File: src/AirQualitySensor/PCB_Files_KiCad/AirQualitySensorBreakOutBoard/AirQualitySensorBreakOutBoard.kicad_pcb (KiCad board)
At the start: 2 copper layers, 113.8 x 36 mm, 23 parts, among them J1 Conn_01x02_Male, J2 Conn_01x02_Male, J3 Conn_01x02_Male, J4 Conn_01x07_Male, Q1 IRLB8721PBF, U1 PMS5003, U2 PMS5003, U3 SPS30, U4 SHT31, U6 lilygo-ttgo-t-sim7000g-esp32-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

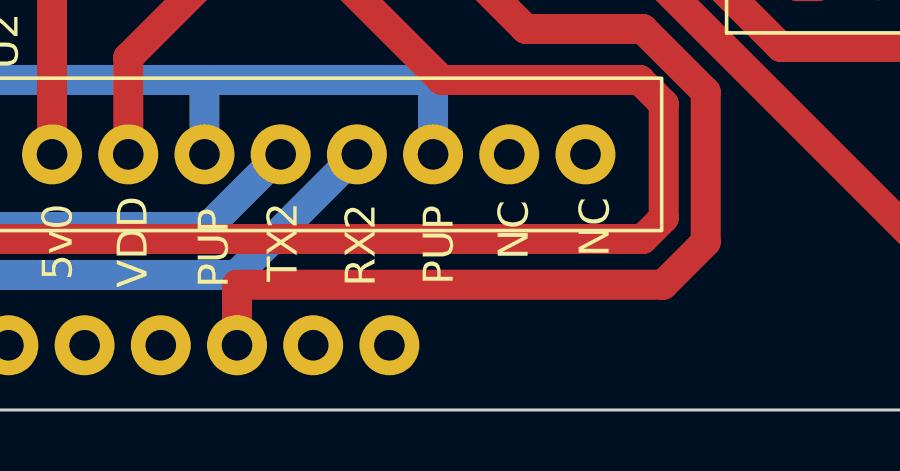
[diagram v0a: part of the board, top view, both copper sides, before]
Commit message: Fixed bug aqs
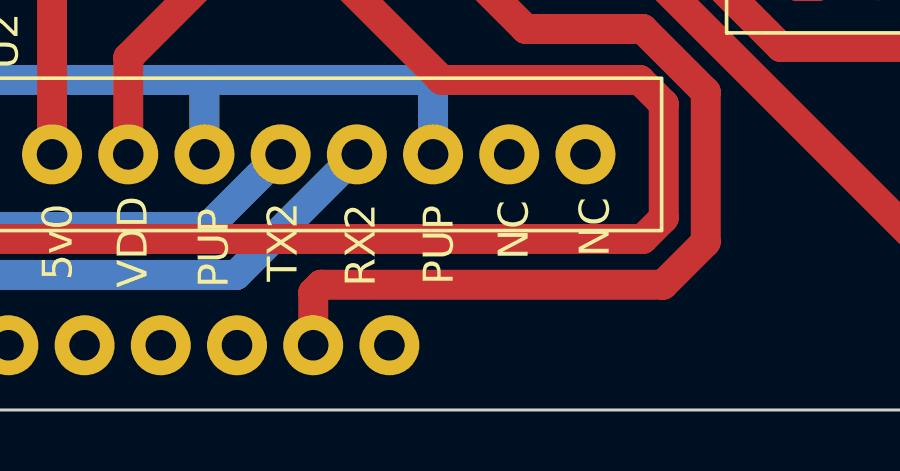
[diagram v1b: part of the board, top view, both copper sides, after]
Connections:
- U6 pad 12: unconnected-(U6-Pad12) -> VDD_EN
- U6 pad 13: VDD_EN -> unconnected-(U6-Pad13)
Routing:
- net VDD_EN: track 34.6 -> 31.9 mm
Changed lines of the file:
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@@
   (net 7 "unconnected-(U6-Pad03)")
   (net 8 "unconnected-(U6-Pad04)")
-  (net 9 "unconnected-(U6-Pad12)")
+  (net 9 "unconnected-(U6-Pad13)")
   (net 10 "unconnected-(U6-Pad14)")
   (net 11 "unconnected-(U6-Pad15)")
@@
       (net 34 "SPI_SS") (pinfunction "SPI__SS") (pintype "input"))
     (pad "12" thru_hole circle (at -14.12 -4.6 90) (size 2 2) (drill 1.02) (layers *.Cu *.Mask)
-      (net 9 "unconnected-(U6-Pad12)") (pinfunction "12") (pintype "input"))
+      (net 38 "VDD_EN") (pinfunction "12") (pintype "input"))
     (pad "13" thru_hole circle (at -14.12 -7.14 90) (size 2 2) (drill 1.02) (layers *.Cu *.Mask)
-      (net 38 "VDD_EN") (pinfunction "13") (pintype "input"))
+      (net 9 "unconnected-(U6-Pad13)") (pinfunction "13") (pintype "input"))
     (pad "14" thru_hole circle (at -14.12 -9.68 90) (size 2 2) (drill 1.02) (layers *.Cu *.Mask)
       (net 10 "unconnected-(U6-Pad14)") (pinfunction "14") (pintype "input"))
@@
   (segment (start 39.86 20.5) (end 38.085 18.725) (width 1) (layer "F.Cu") (net 37))
   (segment (start 38.085 18.725) (end 38.085 16.663353) (width 1) (layer "F.Cu") (net 37))
-  (segment (start 62.5 33.51) (end 62.5 33.6) (width 1) (layer "F.Cu") (net 38))
+  (segment (start 71.6 43.8) (end 70.174649 45.225351) (width 1) (layer "F.Cu") (net 38))
+  (segment (start 62.5 33.6) (end 65.6 36.7) (width 1) (layer "F.Cu") (net 38))
   (segment (start 71.6 38.8) (end 71.6 43.8) (width 1) (layer "F.Cu") (net 38))
-  (segment (start 69.5 36.7) (end 71.6 38.8) (width 1) (layer "F.Cu") (net 38))
-  (segment (start 70.174649 45.225351) (end 55.974649 45.225351) (width 1) (layer "F.Cu") (net 38))
   (segment (start 65.6 36.7) (end 69.5 36.7) (width 1) (layer "F.Cu") (net 38))
-  (segment (start 55.974649 45.225351) (end 55.974649 47.243002) (width 1) (layer "F.Cu") (net 38))
-  (segment (start 62.5 33.6) (end 65.6 36.7) (width 1) (layer "F.Cu") (net 38))
-  (segment (start 71.6 43.8) (end 70.174649 45.225351) (width 1) (layer "F.Cu") (net 38))
+  (segment (start 62.5 33.51) (end 62.5 33.6) (width 1) (layer "F.Cu") (net 38))
+  (segment (start 69.5 36.7) (end 71.6 38.8) (width 1) (layer "F.Cu") (net 38))
+  (segment (start 58.514649 45.485351) (end 58.514649 47.243002) (width 1) (layer "F.Cu") (net 38))
+  (segment (start 58.774649 45.225351) (end 58.514649 45.485351) (width 1) (layer "F.Cu") (net 38))
+  (segment (start 70.174649 45.225351) (end 58.774649 45.225351) (width 1) (layer "F.Cu") (net 38))
 )
